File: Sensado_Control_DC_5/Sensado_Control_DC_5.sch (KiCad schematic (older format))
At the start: 104 parts, among them J1 Jumper, J2 Jumper, J3 Jumper, P1 R_FUENTE_CON, P10 GPIO, P11 TOR_4, P12 TOR_2, P13 TOR_1, P14 TOR_3, P2 I_+, P3 I_-, P4 POWER, P5 RS-232, P6 I2C, P7 SPI, P8 GND_REG, P9 RESET, Q1 NMOS, Q10 PMOS, Q11 NMOS, Q12 NMOS, Q13 NMOS, Q14 PMOS, Q15 PMOS, Q16 PMOS, Q2 NMOS, Q3 NMOS, Q4 NMOS, Q5 NMOS, Q6 PMOS, Q7 PMOS, Q8 PMOS, Q9 PMOS, U1 Atmega328PA, U2 ACS_712, U3 LD1117S50TR_FINAL, Y1 XRCHA_16M

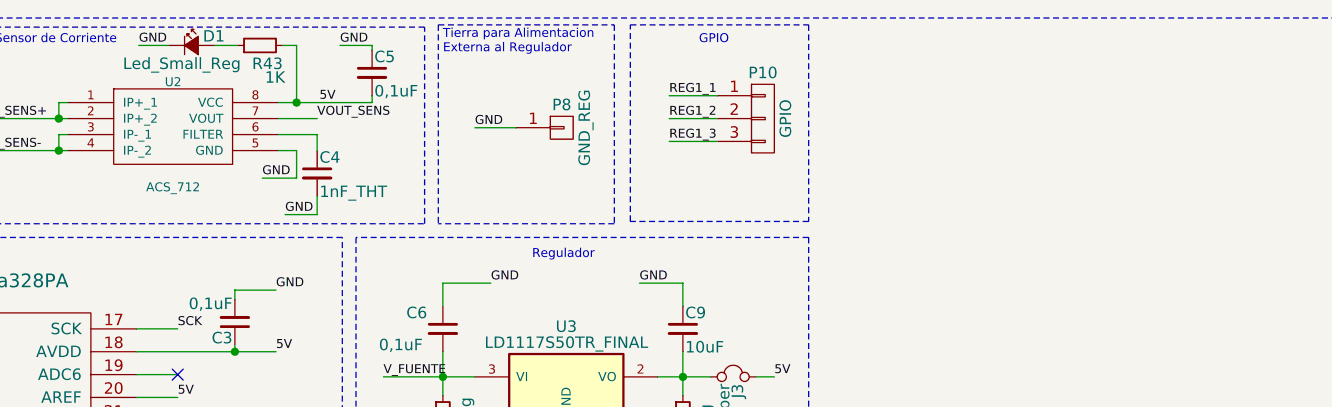
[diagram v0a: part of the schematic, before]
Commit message: Version para placa
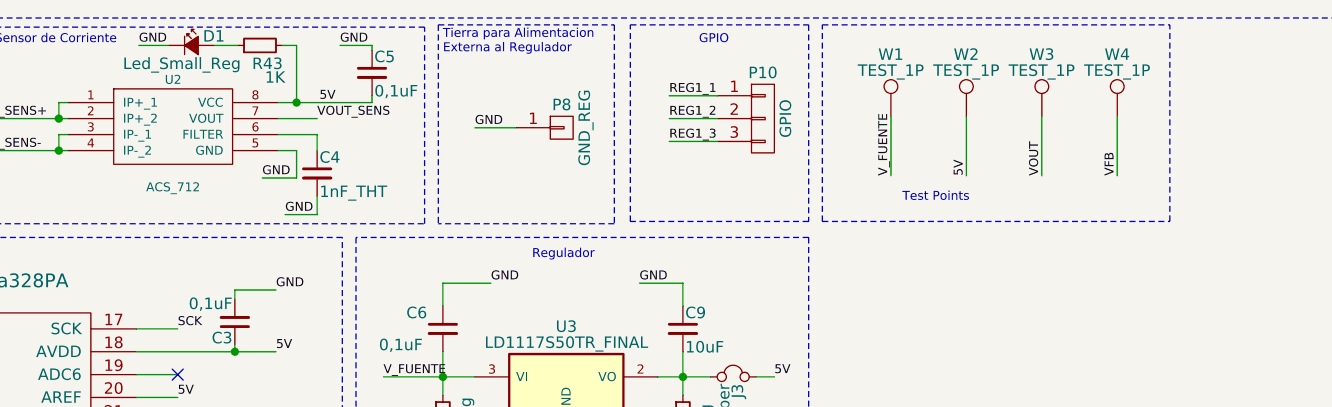
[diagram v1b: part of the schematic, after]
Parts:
- added W1, W2, W3, W4: TEST_1P, Measurement_Points:Measurement_Point_Round-TH_Small, symbol TEST_1P
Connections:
- net 5V: now also W2.1
- net VFB: now also W4.1
- net VOUT: now also W3.1
- net V_FUENTE: now also W1.1
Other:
- note added: "Test Points"
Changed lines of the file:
@@
 In Sensor de Corriente
-$Comp
-L ACS_712 U2
-U 1 1 59D369E2
-P 4500 1040
-F 0 "U2" H 4500 1260 39  0000 C CNN
-F 1 "ACS_712" H 4500 800 39  0000 C CNN
-F 2 "Housings_SOIC:SOIC-8_3.9x4.9mm_Pitch1.27mm" H 4500 1270 39  0001 C CNN
-F 3 "" H 4500 1270 39  0000 C CNN
-	1    4500 1040
-	1    0    0    -1
-$EndComp
 $Comp
 L 0,1uF C5
@@
 NoConn ~ 5600 5450
 NoConn ~ 5960 5160
+$Comp
+L ACS_712 U2
+U 1 1 59D461A2
+P 4500 1040
+F 0 "U2" H 4500 1270 39  0000 C CNN
+F 1 "ACS_712" H 4500 800 39  0000 C CNN
+F 2 "Housings_SOIC:SOIC-8_3.9x4.9mm_Pitch1.27mm" H 4500 1270 39  0001 C CNN
+F 3 "" H 4500 1270 39  0000 C CNN
+	1    4500 1040
+	1    0    0    -1
+$EndComp
+Wire Notes Line
+	7340 1430 7340 570
+Wire Notes Line
+	7340 570  8860 570
+Wire Notes Line
+	7340 1430 8860 1430
+$Comp
+L TEST_1P W1
+U 1 1 59D92BFD
+P 7640 970
+F 0 "W1" H 7640 1240 50  0000 C CNN
+F 1 "TEST_1P" H 7640 1170 50  0000 C CNN
+F 2 "Measurement_Points:Measurement_Point_Round-TH_Small" H 7840 970 50  0001 C CNN
+F 3 "" H 7840 970 50  0000 C CNN
+	1    7640 970
+	1    0    0    -1
+$EndComp
+$Comp
+L TEST_1P W2
+U 1 1 59D92DB8
+P 7970 970
+F 0 "W2" H 7970 1240 50  0000 C CNN
+F 1 "TEST_1P" H 7970 1170 50  0000 C CNN
+F 2 "Measurement_Points:Measurement_Point_Round-TH_Small" H 8170 970 50  0001 C CNN
+F 3 "" H 8170 970 50  0000 C CNN
+	1    7970 970
+	1    0    0    -1
+$EndComp
+$Comp
+L TEST_1P W3
+U 1 1 59D92EE0
+P 8300 970
+F 0 "W3" H 8300 1240 50  0000 C CNN
+F 1 "TEST_1P" H 8300 1170 50  0000 C CNN
+F 2 "Measurement_Points:Measurement_Point_Round-TH_Small" H 8500 970 50  0001 C CNN
+F 3 "" H 8500 970 50  0000 C CNN
+	1    8300 970
+	1    0    0    -1
+$EndComp
+$Comp
+L TEST_1P W4
+U 1 1 59D92EE6
+P 8630 970
+F 0 "W4" H 8630 1240 50  0000 C CNN
+F 1 "TEST_1P" H 8630 1170 50  0000 C CNN
+F 2 "Measurement_Points:Measurement_Point_Round-TH_Small" H 8830 970 50  0001 C CNN
+F 3 "" H 8830 970 50  0000 C CNN
+	1    8630 970
+	1    0    0    -1
+$EndComp
+Wire Wire Line
+	7640 970  7640 1230
+Wire Wire Line
+	7970 970  7970 1230
+Wire Wire Line
+	8300 970  8300 1230
+Wire Wire Line
+	8630 970  8630 1230
+Wire Notes Line
+	8860 1430 8860 570
+Text Label 7640 1230 1    39   ~ 0
+V_FUENTE
+Text Label 7970 1230 1    39   ~ 0
+5V
+Text Label 8300 1230 1    39   ~ 0
+VOUT
+Text Label 8630 1230 1    39   ~ 0
+VFB
+Text Notes 7690 1350 0    39   ~ 0
+Test Points
 $EndSCHEMATC
